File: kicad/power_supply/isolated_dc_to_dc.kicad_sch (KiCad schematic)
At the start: 23 parts, among them U201 LM25184NGUR, U202 750313445

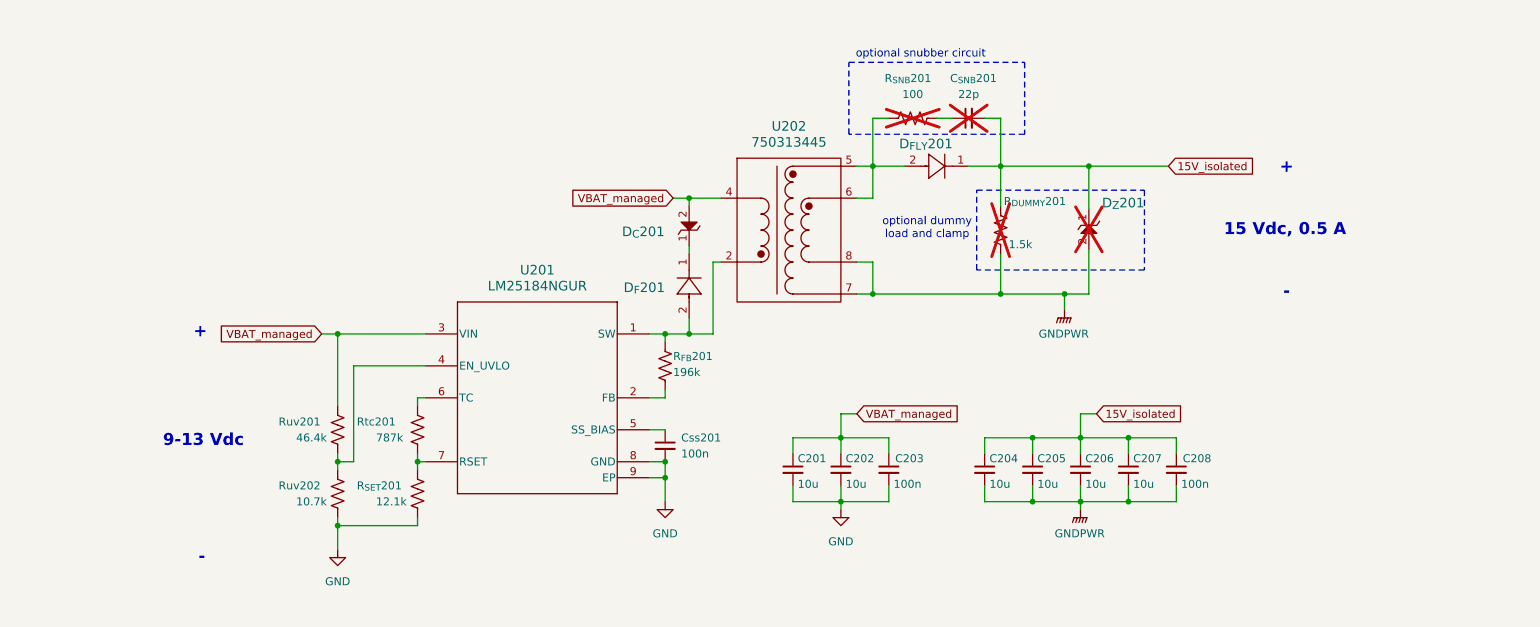
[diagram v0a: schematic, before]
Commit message: updated psu
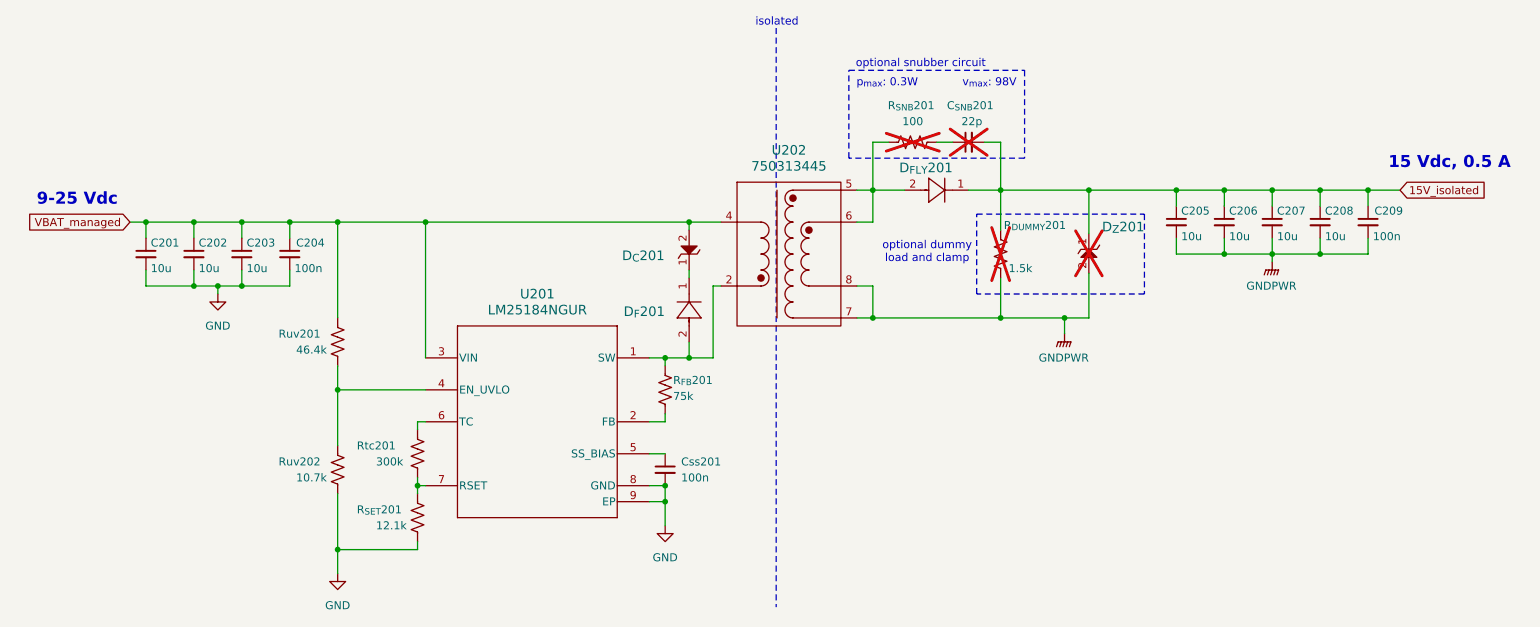
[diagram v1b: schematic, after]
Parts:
- added C209: 100n, Capacitor_SMD:C_0402_1005Metric, symbol Device:C_Small
- C203, C208: value 100n -> 10u; footprint Capacitor_SMD:C_0402_1005Metric -> Capacitor_SMD:C_1206_3216Metric
- C204: value 10u -> 100n; footprint Capacitor_SMD:C_1206_3216Metric -> Capacitor_SMD:C_0402_1005Metric
- R_{FB}201: value 196k -> 75k
- Rtc201: value 787k -> 300k
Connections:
- net 15V_isolated: now also C209.1; no longer C204.1
- net GND: now also C204.2
- net GNDPWR: now also C209.2; no longer C204.2
- net VBAT_managed: now also C204.1
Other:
- note added: "9-25 Vdc"
- note added: "isolated"
- note added: "p_{max}: 0.3W"
- note added: "v_{max}: 98V"
- note removed: "+"
- note removed: "-"
- note removed: "9-13 Vdc"
- moved on the sheet: C_{SNB}201, Css201, D_{C}201, D_{FLY}201, D_{F}201, D_{Z}201, R_{DUMMY}201, R_{FB}201, R_{SET}201, R_{SNB}201, Rtc201, Ruv201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
